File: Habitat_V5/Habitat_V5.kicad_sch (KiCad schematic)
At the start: 98 parts, among them J1 Conn_01x04_Socket, J2 Conn_01x03_Socket, J3 Conn_01x04_Socket, J4 Conn_01x04_Socket, J5 Conn_01x03_Socket, K1 Relay_SPDT, Q1 PMOS, Q2 2N7002K, U1 XL1509-5V, U2 AP2112K-3.3, U3 PC817, U6 ESP32-S3-WROOM-1

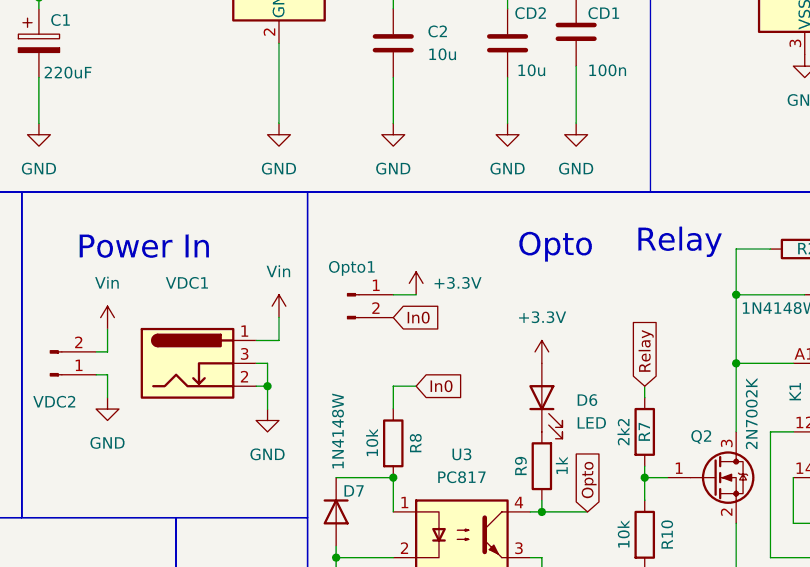
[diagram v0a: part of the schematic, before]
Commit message: Files for production
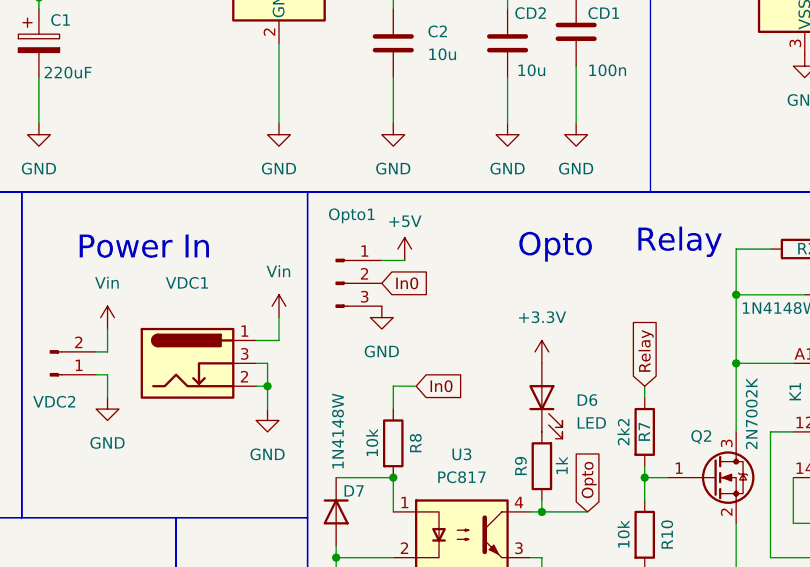
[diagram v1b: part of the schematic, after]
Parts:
- Opto1: value Conn_01x02_Pin -> Conn_01x03_Pin; footprint Connector_Phoenix_MSTB:PhoenixContact_MSTBA_2,5_2-G-5,08_1x02_P5.08mm_Horizontal -> Connector_Phoenix_MSTB:PhoenixContact_MSTBA_2,5_3-G-5,08_1x03_P5.08mm_Horizontal; symbol Connector:Conn_01x02_Pin -> Connector:Conn_01x03_Pin
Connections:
- net +3.3V: no longer Opto1.1 (Pin_1)
- net +5V: now also Opto1.1 (Pin_1)
- net GND: now also Opto1.3 (Pin_3)
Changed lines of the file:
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@@
 	(wire
 		(pts
-			(xy 130.81 68.58) (xy 128.27 68.58)
+			(xy 129.54 64.77) (xy 127 64.77)
 		)
 		(stroke
@@
 	(global_label "In0"
 		(shape input)
-		(at 128.27 71.12 0)
+		(at 127 67.31 0)
 		(fields_autoplaced yes)
 		(effects
@@
 		)
 		(property "Intersheetrefs" "${INTERSHEET_REFS}"
-			(at 134.2185 71.12 0)
+			(at 132.9485 67.31 0)
 			(effects
 				(font
@@
 	)
 	(symbol
-		(lib_id "power:+3.3V")
-		(at 130.81 68.58 0)
-		(unit 1)
-		(exclude_from_sim no)
-		(in_bom yes)
-		(on_board yes)
-		(dnp no)
-		(property "Reference" "#PWR24"
-			(at 130.81 72.39 0)
-			(effects
-				(font
-					(size 1.27 1.27)
-				)
-				(hide yes)
-			)
-		)
-		(property "Value" "+3.3V"
-			(at 135.382 67.31 0)
-			(effects
-				(font
-					(size 1.27 1.27)
-				)
-			)
-		)
-		(property "Footprint" ""
-			(at 130.81 68.58 0)
-			(effects
-				(font
-					(size 1.27 1.27)
-				)
-				(hide yes)
-			)
-		)
-		(property "Datasheet" ""
-			(at 130.81 68.58 0)
-			(effects
-				(font
-					(size 1.27 1.27)
-				)
-				(hide yes)
-			)
-		)
-		(property "Description" "Power symbol creates a global label with name \"+3.3V\""
-			(at 130.81 68.58 0)
-			(effects
-				(font
-					(size 1.27 1.27)
-				)
-				(hide yes)
-			)
-		)
-		(pin "1"
-		)
-		(instances
-			(project "Habitat_V5"
-				(path "/5da8ef61-9b4a-4ae5-94b1-3a318860cb02"
-					(reference "#PWR24")
-					(unit 1)
-				)
-			)
-		)
-	)
-	(symbol
 		(lib_id "Device:C_Polarized")
 		(at 78.74 187.96 0)
@@
 	)
 	(symbol
-		(lib_id "Connector:Conn_01x02_Pin")
-		(at 123.19 68.58 0)
+		(lib_id "Connector:Conn_01x03_Pin")
+		(at 121.92 67.31 0)
 		(unit 1)
 		(exclude_from_sim no)
@@
 		(dnp no)
 		(property "Reference" "Opto1"
-			(at 123.698 65.532 0)
+			(at 123.698 59.69 0)
 			(effects
 				(font
@@
 			)
 		)
-		(property "Value" "Conn_01x02_Pin"
-			(at 123.825 66.04 0)
+		(property "Value" "Conn_01x03_Pin"
+			(at 122.555 64.77 0)
 			(effects
 				(font
@@
 			)
 		)
-		(property "Footprint" "Connector_Phoenix_MSTB:PhoenixContact_MSTBA_2,5_2-G-5,08_1x02_P5.08mm_Horizontal"
-			(at 123.19 68.58 0)
+		(property "Footprint" "Connector_Phoenix_MSTB:PhoenixContact_MSTBA_2,5_3-G-5,08_1x03_P5.08mm_Horizontal"
+			(at 121.92 67.31 0)
 			(effects
 				(font
@@
 		)
 		(property "Datasheet" "~"
-			(at 123.19 68.58 0)
+			(at 121.92 67.31 0)
 			(effects
 				(font
@@
 			)
 		)
-		(property "Description" "Generic connector, single row, 01x02, script generated"
-			(at 123.19 68.58 0)
+		(property "Description" "Generic connector, single row, 01x03, script generated"
+			(at 121.92 67.31 0)
 			(effects
 				(font
@@
 		)
 		(property "LCSC" "1"
-			(at 123.19 68.58 0)
+			(at 121.92 67.31 0)
 			(effects
 				(font
@@
 		)
 		(property "ASSEMBLY" ""
-			(at 123.19 68.58 0)
+			(at 121.92 67.31 0)
 			(effects
 				(font
@@
 		)
 		(property "PART NUMBER" ""
-			(at 123.19 68.58 0)
+			(at 121.92 67.31 0)
 			(effects
 				(font
@@
 		)
 		(property "SUPPLIER 1" ""
-			(at 123.19 68.58 0)
+			(at 121.92 67.31 0)
 			(effects
 				(font
@@
 		)
 		(property "SUPPLIER 2" ""
-			(at 123.19 68.58 0)
+			(at 121.92 67.31 0)
 			(effects
 				(font
@@
 		)
 		(property "SUPPLIER 3" ""
-			(at 123.19 68.58 0)
+			(at 121.92 67.31 0)
 			(effects
 				(font
@@
 		)
 		(property "SUPPLIER PART NUMBER 1" ""
-			(at 123.19 68.58 0)
+			(at 121.92 67.31 0)
 			(effects
 				(font
@@
 		)
 		(property "SUPPLIER PART NUMBER 2" ""
-			(at 123.19 68.58 0)
+			(at 121.92 67.31 0)
 			(effects
 				(font
@@
 		)
 		(property "SUPPLIER PART NUMBER 3" ""
-			(at 123.19 68.58 0)
+			(at 121.92 67.31 0)
 			(effects
 				(font
@@
 		)
 		(property "TYPE" ""
-			(at 123.19 68.58 0)
+			(at 121.92 67.31 0)
 			(effects
 				(font
@@
 		(pin "1"
 		)
+		(pin "3"
+		)
 		(instances
 			(project "Habitat_V5"
@@
 	)
 	(symbol
+		(lib_id "power:GND")
+		(at 127 69.85 0)
+		(unit 1)
+		(exclude_from_sim no)
+		(in_bom yes)
+		(on_board yes)
+		(dnp no)
+		(fields_autoplaced yes)
+		(property "Reference" "#PWR145"
+			(at 127 76.2 0)
+			(effects
+				(font
+					(size 1.27 1.27)
+				)
+				(hide yes)
+			)
+		)
+		(property "Value" "GND"
+			(at 127 74.93 0)
+			(effects
+				(font
+					(size 1.27 1.27)
+				)
+			)
+		)
+		(property "Footprint" ""
+			(at 127 69.85 0)
+			(effects
+				(font
+					(size 1.27 1.27)
+				)
+				(hide yes)
+			)
+		)
+		(property "Datasheet" ""
+			(at 127 69.85 0)
+			(effects
+				(font
+					(size 1.27 1.27)
+				)
+				(hide yes)
+			)
+		)
+		(property "Description" "Power symbol creates a global label with name \"GND\" , ground"
+			(at 127 69.85 0)
+			(effects
+				(font
+					(size 1.27 1.27)
+				)
+				(hide yes)
+			)
+		)
+		(pin "1"
+		)
+		(instances
+			(project "Habitat_V5"
+				(path "/5da8ef61-9b4a-4ae5-94b1-3a318860cb02"
+					(reference "#PWR145")
+					(unit 1)
+				)
+			)
+		)
+	)
+	(symbol
 		(lib_id "Device:D_Zener")
 		(at 31.75 38.1 180)
@@
 					(unit 1)
 				)
+			)
+		)
+	)
+	(symbol
+		(lib_id "power:+5V")
+		(at 129.54 64.77 0)
+		(unit 1)
+		(exclude_from_sim no)
+		(in_bom yes)
+		(on_board yes)
+		(dnp no)
+		(property "Reference" "#PWR24"
+			(at 129.54 68.58 0)
+			(effects
+				(font
+					(size 1.27 1.27)
+				)
+				(hide yes)
+			)
+		)
+		(property "Value" "+5V"
+			(at 129.54 60.452 0)
+			(effects
+				(font
+					(size 1.27 1.27)
+				)
+			)
+		)
+		(property "Footprint" ""
+			(at 129.54 64.77 0)
+			(effects
+				(font
+					(size 1.27 1.27)
+				)
+				(hide yes)
+			)
+		)
+		(property "Datasheet" ""
+			(at 129.54 64.77 0)
+			(effects
+				(font
+					(size 1.27 1.27)
+				)
+				(hide yes)
+			)
+		)
+		(property "Description" "Power symbol creates a global label with name \"+5V\""
+			(at 129.54 64.77 0)
+			(effects
+				(font
+					(size 1.27 1.27)
+				)
+				(hide yes)
+			)
+		)
+		(pin "1"
+		)
+		(instances
+			(project "Habitat_V5"
+				(path "/5da8ef61-9b4a-4ae5-94b1-3a318860cb02"
+					(reference "#PWR24")
+					(unit 1)
+				)
